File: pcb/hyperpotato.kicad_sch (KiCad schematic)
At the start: 46 parts, among them J1 Conn_01x02_Socket, J2 Conn_01x03_Pin, Q1 AO3401A, SW1 SW_Push_45deg, SW10 SW_Push_45deg, SW11 SW_Push_45deg, SW12 SW_Push_45deg, SW13 SW_Push_45deg, SW14 SW_SPDT, SW15 SW_Push, SW2 SW_Push_45deg, SW3 SW_Push_45deg, SW4 SW_Push_45deg, SW5 SW_Push_45deg, SW6 SW_Push_45deg, SW7 SW_Push_45deg, SW8 SW_Push_45deg, SW9 SW_Push_45deg, U1 Seeeduino Xiao nRF52840, U2 SK8707-01-SENSOR, U3 SK8707-01, U4 DRV2605LDGS, U5 74HC595

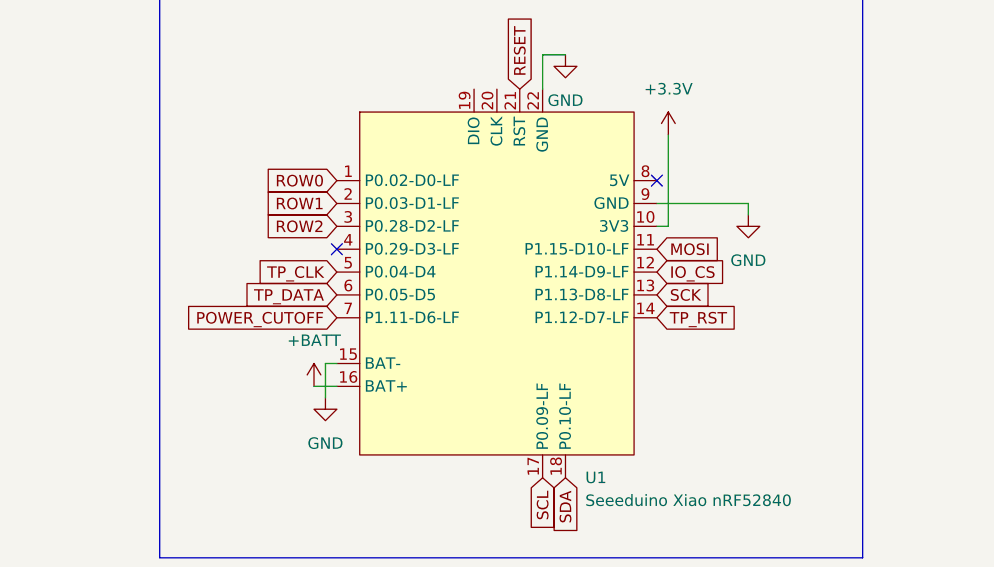
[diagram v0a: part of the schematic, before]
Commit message: Good progress on routing
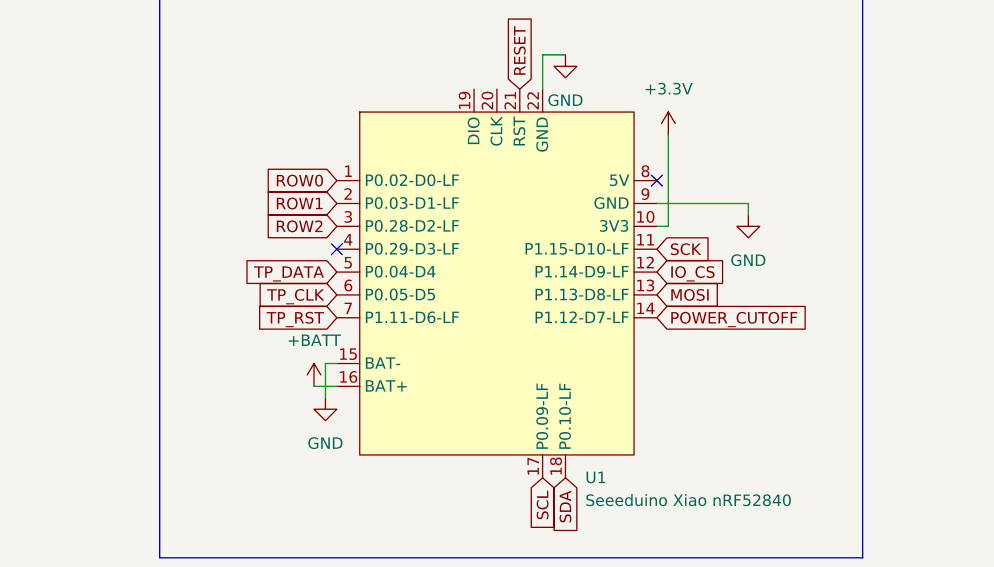
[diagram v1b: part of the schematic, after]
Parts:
- U5: footprint ssbb_parts_reversible:SOIC-16_3.9x9.9mm_P1.27mm_reversible -> ssbb_parts_reversible:TSSOP-16_4.4x5mm_P0.65mm_reversible
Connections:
- net MOSI: now also U1.13 (P1.13-D8-LF); no longer U1.11 (P1.15-D10-LF)
- net POWER_CUTOFF: now also U1.14 (P1.12-D7-LF); no longer U1.7 (P1.11-D6-LF)
- net SCK: now also U1.11 (P1.15-D10-LF); no longer U1.13 (P1.13-D8-LF)
- net TP_CLK: now also U1.6 (P0.05-D5); no longer U1.5 (P0.04-D4)
- net TP_DATA: now also U1.5 (P0.04-D4); no longer U1.6 (P0.05-D5)
- net TP_RST: now also U1.7 (P1.11-D6-LF); no longer U1.14 (P1.12-D7-LF)
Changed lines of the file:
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@@
 		)
 	)
-	(global_label "IO_CS"
+	(global_label "SCL"
 		(shape input)
-		(at 181.61 182.88 180)
+		(at 86.36 275.59 270)
 		(fields_autoplaced yes)
 		(effects
@@
 		)
 		(property "Intersheetrefs" "${INTERSHEET_REFS}"
-			(at 173.3218 182.88 0)
+			(at 86.36 282.0828 90)
 			(effects
 				(font
@@
 		)
 	)
-	(global_label "SCK"
+	(global_label "IO_CS"
 		(shape input)
-		(at 99.06 255.27 0)
+		(at 181.61 182.88 180)
 		(fields_autoplaced yes)
 		(effects
@@
 				(size 1.27 1.27)
 			)
-			(justify left)
+			(justify right)
 		)
 		(property "Intersheetrefs" "${INTERSHEET_REFS}"
-			(at 105.7947 255.27 0)
+			(at 173.3218 182.88 0)
 			(effects
 				(font
 					(size 1.27 1.27)
 				)
-				(justify left)
+				(justify right)
 				(hide yes)
 			)
@@
 		)
 	)
+	(global_label "SCK"
+		(shape input)
+		(at 99.06 250.19 0)
+		(fields_autoplaced yes)
+		(effects
+			(font
+				(size 1.27 1.27)
+			)
+			(justify left)
+		)
+		(property "Intersheetrefs" "${INTERSHEET_REFS}"
+			(at 105.7947 250.19 0)
+			(effects
+				(font
+					(size 1.27 1.27)
+				)
+				(justify left)
+				(hide yes)
+			)
+		)
+	)
 	(global_label "RESET"
 		(shape input)
@@
 		)
 	)
-	(global_label "POWER_CUTOFF"
+	(global_label "TP_CLK"
 		(shape input)
-		(at 63.5 257.81 180)
+		(at 63.5 255.27 180)
 		(fields_autoplaced yes)
 		(effects
@@
 		)
 		(property "Intersheetrefs" "${INTERSHEET_REFS}"
-			(at 46.0005 257.81 0)
+			(at 53.7415 255.27 0)
 			(effects
 				(font
@@
 		)
 	)
-	(global_label "MOSI"
-		(shape input)
-		(at 99.06 250.19 0)
-		(fields_autoplaced yes)
-		(effects
-			(font
-				(size 1.27 1.27)
-			)
-			(justify left)
-		)
-		(property "Intersheetrefs" "${INTERSHEET_REFS}"
-			(at 106.6414 250.19 0)
-			(effects
-				(font
-					(size 1.27 1.27)
-				)
-				(justify left)
-				(hide yes)
-			)
-		)
-	)
-	(global_label "TP_RST"
+	(global_label "RESET"
 		(shape input)
-		(at 99.06 257.81 0)
+		(at 83.82 232.41 90)
 		(fields_autoplaced yes)
 		(effects
@@
 		)
 		(property "Intersheetrefs" "${INTERSHEET_REFS}"
-			(at 108.6975 257.81 0)
+			(at 83.82 223.6797 90)
 			(effects
 				(font
@@
 		)
 	)
-	(global_label "RESET"
+	(global_label "POWER_CUTOFF"
 		(shape input)
-		(at 83.82 232.41 90)
+		(at 110.49 86.36 0)
 		(fields_autoplaced yes)
 		(effects
@@
 		)
 		(property "Intersheetrefs" "${INTERSHEET_REFS}"
-			(at 83.82 223.6797 90)
+			(at 127.9895 86.36 0)
 			(effects
 				(font
@@
 		)
 	)
-	(global_label "POWER_CUTOFF"
+	(global_label "COL4"
 		(shape input)
-		(at 110.49 86.36 0)
+		(at 204.47 175.26 0)
 		(fields_autoplaced yes)
 		(effects
@@
 		)
 		(property "Intersheetrefs" "${INTERSHEET_REFS}"
-			(at 127.9895 86.36 0)
+			(at 212.2933 175.26 0)
 			(effects
 				(font
@@
 		)
 	)
-	(global_label "COL4"
+	(global_label "LED3"
 		(shape input)
-		(at 204.47 175.26 0)
+		(at 204.47 177.8 0)
 		(fields_autoplaced yes)
 		(effects
@@
 		)
 		(property "Intersheetrefs" "${INTERSHEET_REFS}"
-			(at 212.2933 175.26 0)
+			(at 212.1118 177.8 0)
 			(effects
 				(font
@@
 		)
 	)
-	(global_label "LED3"
+	(global_label "MOSI"
 		(shape input)
-		(at 204.47 177.8 0)
+		(at 99.06 255.27 0)
 		(fields_autoplaced yes)
 		(effects
@@
 		)
 		(property "Intersheetrefs" "${INTERSHEET_REFS}"
-			(at 212.1118 177.8 0)
+			(at 106.6414 255.27 0)
 			(effects
 				(font
@@
 		)
 	)
-	(global_label "COL4"
+	(global_label "POWER_CUTOFF"
 		(shape input)
-		(at 81.28 27.94 90)
+		(at 99.06 257.81 0)
 		(fields_autoplaced yes)
 		(effects
@@
 		)
 		(property "Intersheetrefs" "${INTERSHEET_REFS}"
-			(at 81.28 20.1167 90)
+			(at 112.4833 257.81 0)
 			(effects
 				(font
@@
 		)
 	)
-	(global_label "SCL"
+	(global_label "TP_RST"
 		(shape input)
-		(at 86.36 275.59 270)
+		(at 63.5 257.81 180)
 		(fields_autoplaced yes)
 		(effects
@@
 		)
 		(property "Intersheetrefs" "${INTERSHEET_REFS}"
-			(at 86.36 282.0828 90)
+			(at 55.407 257.81 0)
 			(effects
 				(font
@@
 		)
 	)
-	(global_label "TP_CLK"
+	(global_label "COL4"
 		(shape input)
-		(at 139.7 157.48 0)
+		(at 81.28 27.94 90)
 		(fields_autoplaced yes)
 		(effects
@@
 		)
 		(property "Intersheetrefs" "${INTERSHEET_REFS}"
-			(at 149.4585 157.48 0)
+			(at 81.28 20.1167 90)
 			(effects
 				(font
@@
 		)
 	)
-	(global_label "TP_DATA"
+	(global_label "SDA"
 		(shape input)
-		(at 63.5 255.27 180)
+		(at 88.9 275.59 270)
 		(fields_autoplaced yes)
 		(effects
@@
 		)
 		(property "Intersheetrefs" "${INTERSHEET_REFS}"
-			(at 52.8948 255.27 0)
+			(at 88.9 282.1433 90)
 			(effects
 				(font
@@
 		)
 	)
+	(global_label "TP_CLK"
+		(shape input)
+		(at 139.7 157.48 0)
+		(fields_autoplaced yes)
+		(effects
+			(font
+				(size 1.27 1.27)
+			)
+			(justify left)
+		)
+		(property "Intersheetrefs" "${INTERSHEET_REFS}"
+			(at 149.4585 157.48 0)
+			(effects
+				(font
+					(size 1.27 1.27)
+				)
+				(justify left)
+				(hide yes)
+			)
+		)
+	)
 	(global_label "TP_S1"
 		(shape input)
@@
 		)
 	)
-	(global_label "TP_CLK"
-		(shape input)
-		(at 63.5 252.73 180)
-		(fields_autoplaced yes)
-		(effects
-			(font
-				(size 1.27 1.27)
-			)
-			(justify right)
-		)
-		(property "Intersheetrefs" "${INTERSHEET_REFS}"
-			(at 53.7415 252.73 0)
-			(effects
-				(font
-					(size 1.27 1.27)
-				)
-				(justify right)
-				(hide yes)
-			)
-		)
-	)
 	(global_label "LED1"
 		(shape input)
@@
 		)
 	)
-	(global_label "SDA"
+	(global_label "TP_DATA"
 		(shape input)
-		(at 88.9 275.59 270)
+		(at 63.5 252.73 180)
 		(fields_autoplaced yes)
 		(effects
@@
 		)
 		(property "Intersheetrefs" "${INTERSHEET_REFS}"
-			(at 88.9 282.1433 90)
+			(at 52.8948 252.73 0)
 			(effects
 				(font
@@
 			)
 		)
-		(property "Footprint" "ssbb_parts_reversible:SOIC-16_3.9x9.9mm_P1.27mm_reversible"
+		(property "Footprint" "ssbb_parts_reversible:TSSOP-16_4.4x5mm_P0.65mm_reversible"
 			(at 194.31 180.34 0)
 			(effects
